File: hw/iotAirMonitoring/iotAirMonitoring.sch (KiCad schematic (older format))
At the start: 1 part

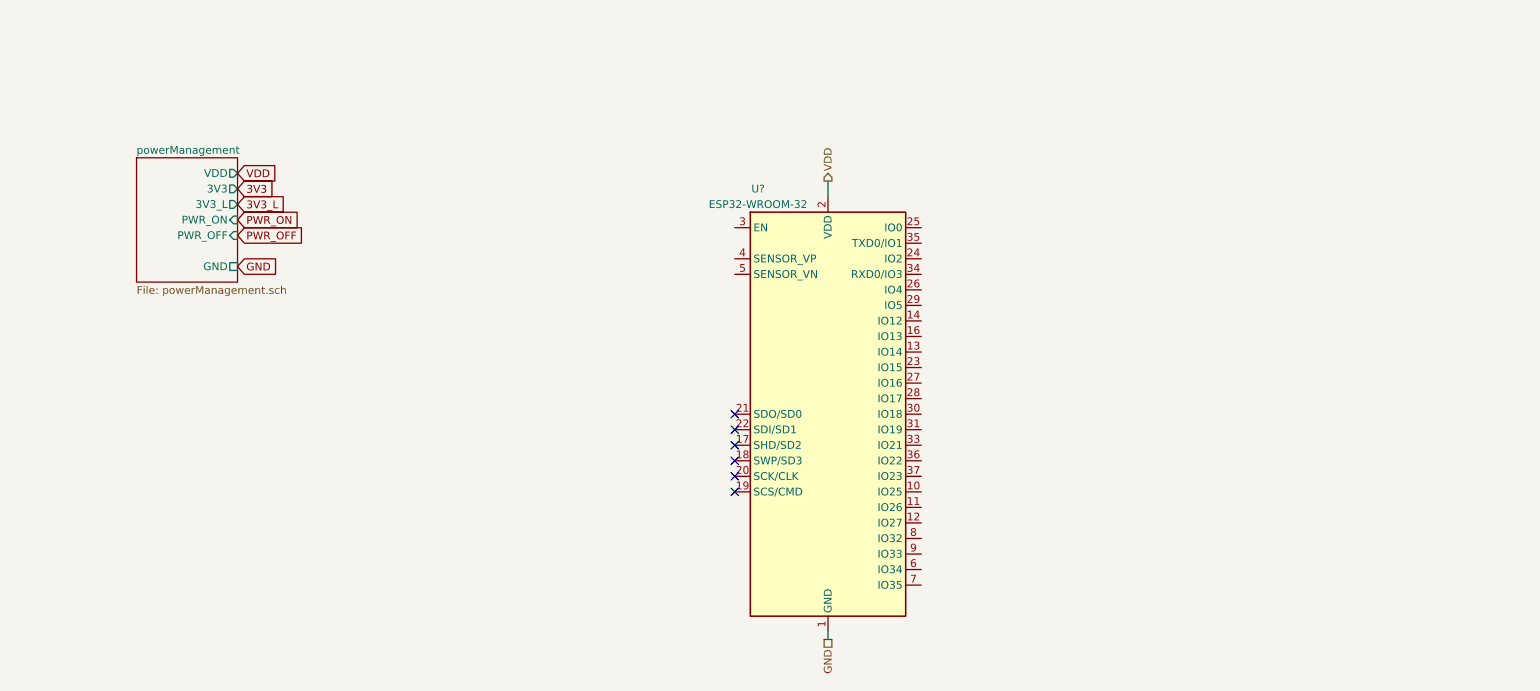
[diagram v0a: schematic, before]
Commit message: More work on schematic
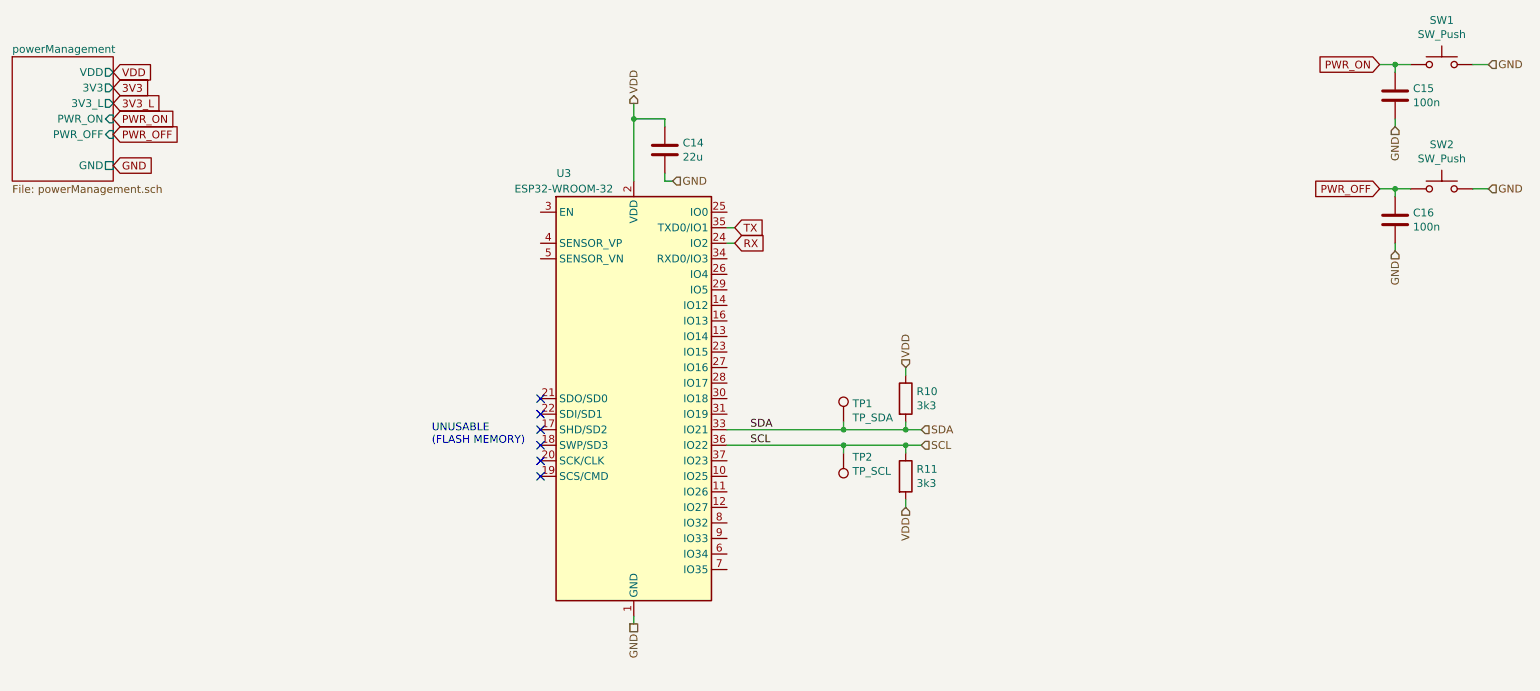
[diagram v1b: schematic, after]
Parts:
- added C14: 22u, Capacitor_SMD:C_0805_2012Metric, symbol Device:C
- added C15, C16: 100n, Capacitor_SMD:C_0402_1005Metric, symbol Device:C
- added R10, R11: 3k3, symbol Device:R
- added SW1, SW2: SW_Push, symbol Switch:SW_Push
- added TP1: TP_SDA, TestPoint:TestPoint_Pad_D1.5mm, symbol Connector:TestPoint
- added TP2: TP_SCL, TestPoint:TestPoint_Pad_D1.5mm, symbol Connector:TestPoint
- gave numbers to parts that had none: 1
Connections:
- net GND: now also C14.2, C15.2, C16.2, SW1.2, SW2.2
- net PWR_OFF: now also C16.1, SW2.1
- net PWR_ON: now also C15.1, SW1.1
- net VDD: now also C14.1, R10.1, R11.2
- net RX: now reaches U3.24 (IO2)
- net SDA: now reaches U3.33 (IO21)
- net SDA: now also R10.2, TP1.1
- net TX: now reaches U3.35 (TXD0/IO1)
- net SCL: now reaches U3.36 (IO22)
- net SCL: now also R11.1, TP2.1
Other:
- note added: "UNUSABLE\n(FLASH MEMORY)"
- moved on the sheet: U3
